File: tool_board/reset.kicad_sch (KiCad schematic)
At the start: 4 parts, among them SW1 SW_Push_Open_Dual

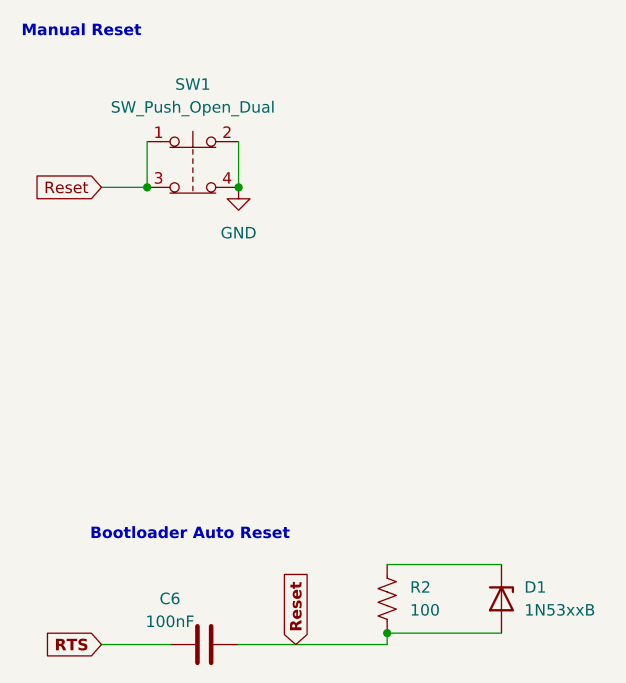
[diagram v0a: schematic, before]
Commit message: message
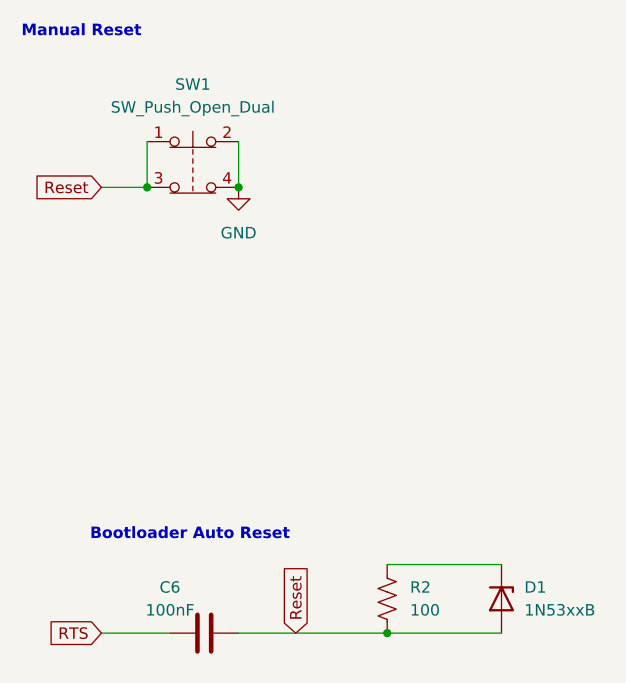
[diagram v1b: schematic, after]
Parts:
- C6: footprint (none) -> Capacitor_SMD:C_0805_2012Metric_Pad1.18x1.45mm_HandSolder
- R2: footprint (none) -> Resistor_SMD:R_0612_1632Metric_Pad1.18x3.40mm_HandSolder
- SW1: footprint (none) -> Button_Switch_SMD:SW_Push_1P1T-SH_NO_CK_KMR2xxG
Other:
- moved on the sheet: C6
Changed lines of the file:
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@@
   (junction (at 85.09 93.98) (diameter 0) (color 0 0 0 0)
   )
-  (wire (pts (xy 68.58 95.25) (xy 85.09 95.25))
+  (wire (pts (xy 68.58 93.98) (xy 85.09 93.98))
     (stroke (width 0) (type default))
   )
@@
     (stroke (width 0) (type default))
   )
-  (wire (pts (xy 53.34 95.25) (xy 60.96 95.25))
+  (wire (pts (xy 53.34 93.98) (xy 60.96 93.98))
     (stroke (width 0) (type default))
   )
@@
     (stroke (width 0) (type default))
   )
-  (wire (pts (xy 85.09 95.25) (xy 85.09 93.98))
-    (stroke (width 0) (type default))
-  )
   (wire (pts (xy 85.09 93.98) (xy 97.79 93.98))
     (stroke (width 0) (type default))
@@
     (effects (font (size 1.27 1.27) (thickness 0.254) bold) (justify left bottom))
   )
-  (global_label "Reset" (shape input) (at 74.93 95.25 90) (fields_autoplaced)
-    (effects (font (size 1.27 1.27) bold) (justify left))
-    (property "Intersheetrefs" "${INTERSHEET_REFS}" (at 74.93 86.5878 90)
+  (global_label "Reset" (shape input) (at 74.93 93.98 90) (fields_autoplaced)
+    (effects (font (size 1.27 1.27)) (justify left))
+    (property "Intersheetrefs" "${INTERSHEET_REFS}" (at 74.93 85.7938 90)
       (effects (font (size 1.27 1.27)) (justify left) hide)
     )
   )
-  (global_label "RTS" (shape input) (at 53.34 95.25 180) (fields_autoplaced)
-    (effects (font (size 1.27 1.27) bold) (justify right))
-    (property "Intersheetrefs" "${INTERSHEET_REFS}" (at 46.4317 95.25 0)
+  (global_label "RTS" (shape input) (at 53.34 93.98 180) (fields_autoplaced)
+    (effects (font (size 1.27 1.27)) (justify right))
+    (property "Intersheetrefs" "${INTERSHEET_REFS}" (at 46.9077 93.98 0)
       (effects (font (size 1.27 1.27)) (justify right) hide)
     )
@@
       (effects (font (size 1.27 1.27)) (justify left))
     )
-    (property "Footprint" "" (at 86.106 90.424 90)
+    (property "Footprint" "Resistor_SMD:R_0612_1632Metric_Pad1.18x3.40mm_HandSolder" (at 86.106 90.424 90)
       (effects (font (size 1.27 1.27)) hide)
     )
@@
       (effects (font (size 1.27 1.27)))
     )
-    (property "Footprint" "" (at 63.5 34.29 0)
+    (property "Footprint" "Button_Switch_SMD:SW_Push_1P1T-SH_NO_CK_KMR2xxG" (at 63.5 34.29 0)
       (effects (font (size 1.27 1.27)) hide)
     )
@@
     )
   )
-  (symbol (lib_id "Device:C") (at 64.77 95.25 270) (unit 1)
+  (symbol (lib_id "Device:C") (at 64.77 93.98 270) (unit 1)
     (in_bom yes) (on_board yes) (dnp no)
-    (property "Reference" "C6" (at 60.96 90.17 90)
+    (property "Reference" "C6" (at 60.96 88.9 90)
       (effects (font (size 1.27 1.27)))
     )
-    (property "Value" "100nF" (at 60.96 92.71 90)
+    (property "Value" "100nF" (at 60.96 91.44 90)
       (effects (font (size 1.27 1.27)))
     )
-    (property "Footprint" "" (at 60.96 96.2152 0)
+    (property "Footprint" "Capacitor_SMD:C_0805_2012Metric_Pad1.18x1.45mm_HandSolder" (at 60.96 94.9452 0)
       (effects (font (size 1.27 1.27)) hide)
     )
-    (property "Datasheet" "~" (at 64.77 95.25 0)
+    (property "Datasheet" "~" (at 64.77 93.98 0)
       (effects (font (size 1.27 1.27)) hide)
     )
